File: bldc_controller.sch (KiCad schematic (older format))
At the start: 147 parts, among them J1 Conn_01x06_Male, J2 Banana_Jack, Q1 FDN340P, Q10 IRLB8721PBF, Q11 IRLB8721PBF, Q2 DMN65D8L-7, Q3 DMN65D8L-7, Q4 2N3904, Q5 IRF4905, Q6 IRLB8721PBF, Q7 IRLB8721PBF, Q8 IRLB8721PBF, Q9 IRLB8721PBF, SW1 1301.9314, SW2 D6C40 F1 LFS, SW3 D6C40 F1 LFS, U1 ATmega328P-PU, U10 IRS2004, U2 74LVC2G08, U3 uA7810, U4 LM7805_TO220, U5 CD4044BE, U6 LM339, U7 MCP601-xP, U8 IRS2004, U9 IRS2004, Y1 9B-16.000MBBK-B

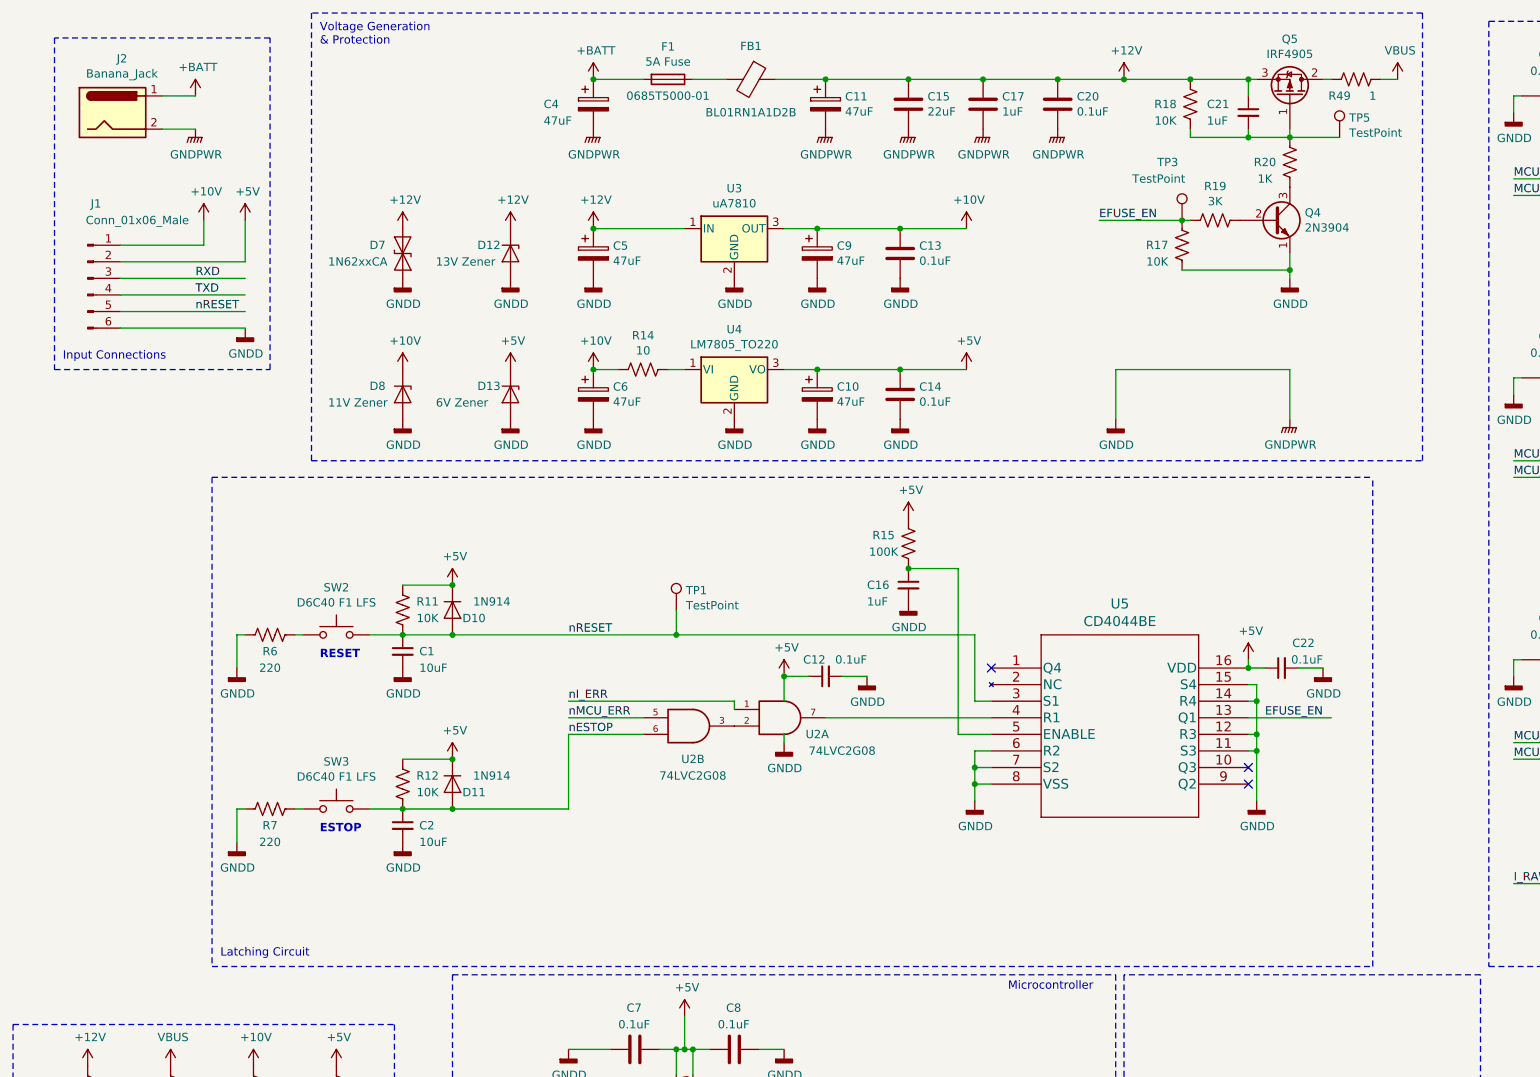
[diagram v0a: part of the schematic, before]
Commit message: Ready for Layout
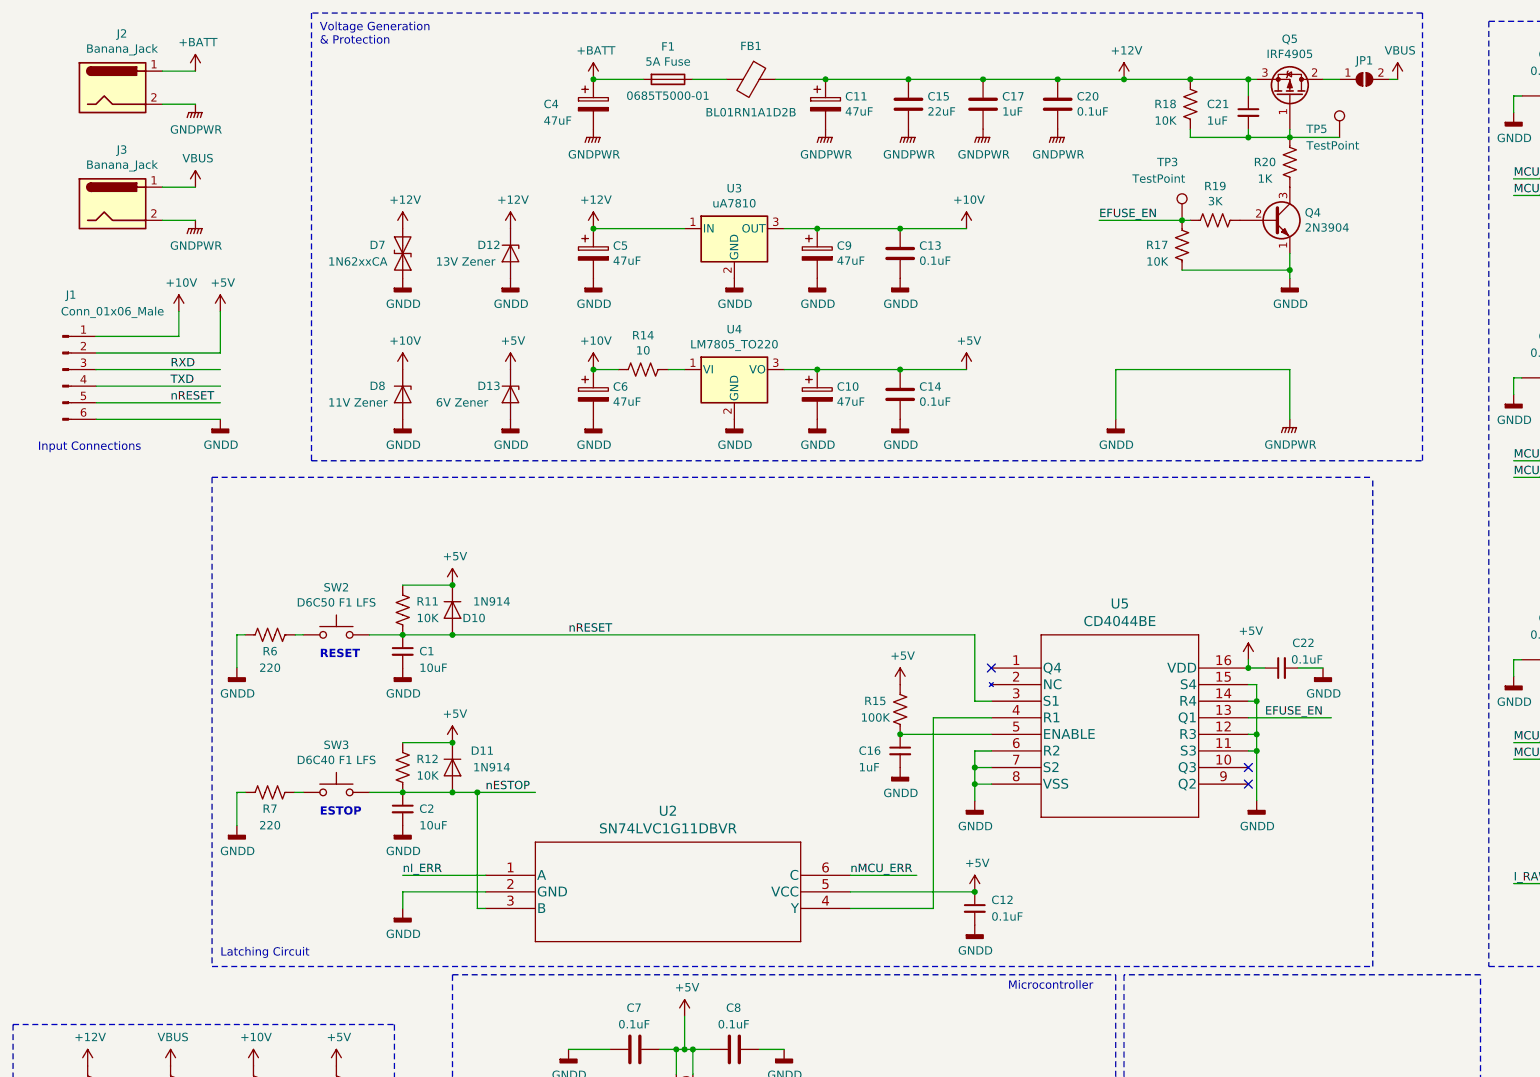
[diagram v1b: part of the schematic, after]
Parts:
- removed R49: 1, symbol Device:R_US
- removed TP1: TestPoint, symbol Connector:TestPoint
- removed U2: 74LVC2G08, symbol 74xGxx:74LVC2G08
- added J3: Banana_Jack, TestPoint:TestPoint_THTPad_D4.0mm_Drill2.0mm, symbol Connector:Barrel_Jack
- added JP1: SolderJumper_2_Open, Jumper:Solder_Jumper_2_Pin_5A, symbol Jumper:SolderJumper_2_Open
- added U2: SN74LVC1G11DBVR, Package_TO_SOT_SMD:SOT-23-6_Handsoldering, symbol SN74LVC1G11DBVR:SN74LVC1G11DBVR
- C1, C12, C13, C14, C15, C16, C17, C18, C19, C2, C20, C21, C22, C23, C24, C25, C26, C27, C28, C29, C3, C30, C31, C32, C33, C7, C8: footprint (none) -> Capacitor_SMD:C_0805_2012Metric_Pad1.15x1.40mm_HandSolder
- C10, C11, C4, C5, C6, C9: footprint (none) -> Capacitor_THT:CP_Radial_D10.0mm_P5.00mm
- D1, D2, D3, D4, D5, D6, D9: footprint (none) -> LED_SMD:LED_0805_2012Metric_Pad1.15x1.40mm_HandSolder
- D12, D13, D8: footprint (none) -> Diode_THT:D_DO-35_SOD27_P7.62mm_Horizontal
- F1: footprint (none) -> Fuse:Fuse_1206_3216Metric_Pad1.42x1.75mm_HandSolder
- FB1: footprint (none) -> Ferrite_THT:Ferrite_Bead_TH
- J1: footprint (none) -> Connector_PinHeader_2.54mm:PinHeader_1x06_P2.54mm_Vertical
- J2: footprint (none) -> TestPoint:TestPoint_THTPad_D4.0mm_Drill2.0mm
- Q1, Q2, Q3: footprint (none) -> Package_TO_SOT_SMD:SOT-23
- R1, R10, R11, R12, R13, R14, R15, R16, R17, R18, R19, R2, R20, R22, R23, R26, R27, R28, R3, R31, R32, R33, R34, R35, R36, R37, R38, R39, R4, R40, R41, R42, R43, R44, R45, R46, R47, R48, R5, R6, R7, R8, R9, RV1: footprint (none) -> Resistor_SMD:R_0805_2012Metric_Pad1.15x1.40mm_HandSolder
- R21, R24, R25, R29, R30: footprint (none) -> Resistor_THT:Power_Resistor_TH
- SW1: footprint (none) -> Button_Switch_SMD:Tactile_Switch_SM
- SW2: value D6C40 F1 LFS -> D6C50 F1 LFS; footprint (none) -> Button_Switch_THT:Pushbutton_Switch_TH
- SW3: footprint (none) -> Button_Switch_THT:Pushbutton_Switch_TH
- TP10, TP11, TP12, TP13, TP14, TP15, TP16, TP17, TP18, TP19, TP2, TP3, TP4, TP5, TP6, TP7, TP8, TP9: footprint (none) -> TestPoint:TestPoint_THTPad_1.0x1.0mm_Drill0.5mm
- U10, U8, U9: footprint (none) -> Package_DIP:DIP-8-16_W7.62mm
- U3: footprint (none) -> Package_TO_SOT_THT:TO-220-3_Vertical
- U5: footprint N16 -> Package_DIP:DIP-16_W7.62mm
- U6: footprint (none) -> Package_DIP:DIP-14_W7.62mm
- Y1: footprint (none) -> Crystal:Crystal_16MHz_TH
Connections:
- wire segments 292 -> 291
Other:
- moved on the sheet: C12, C16, C2, D11, J1, J2, R12, R15, R7, SW3

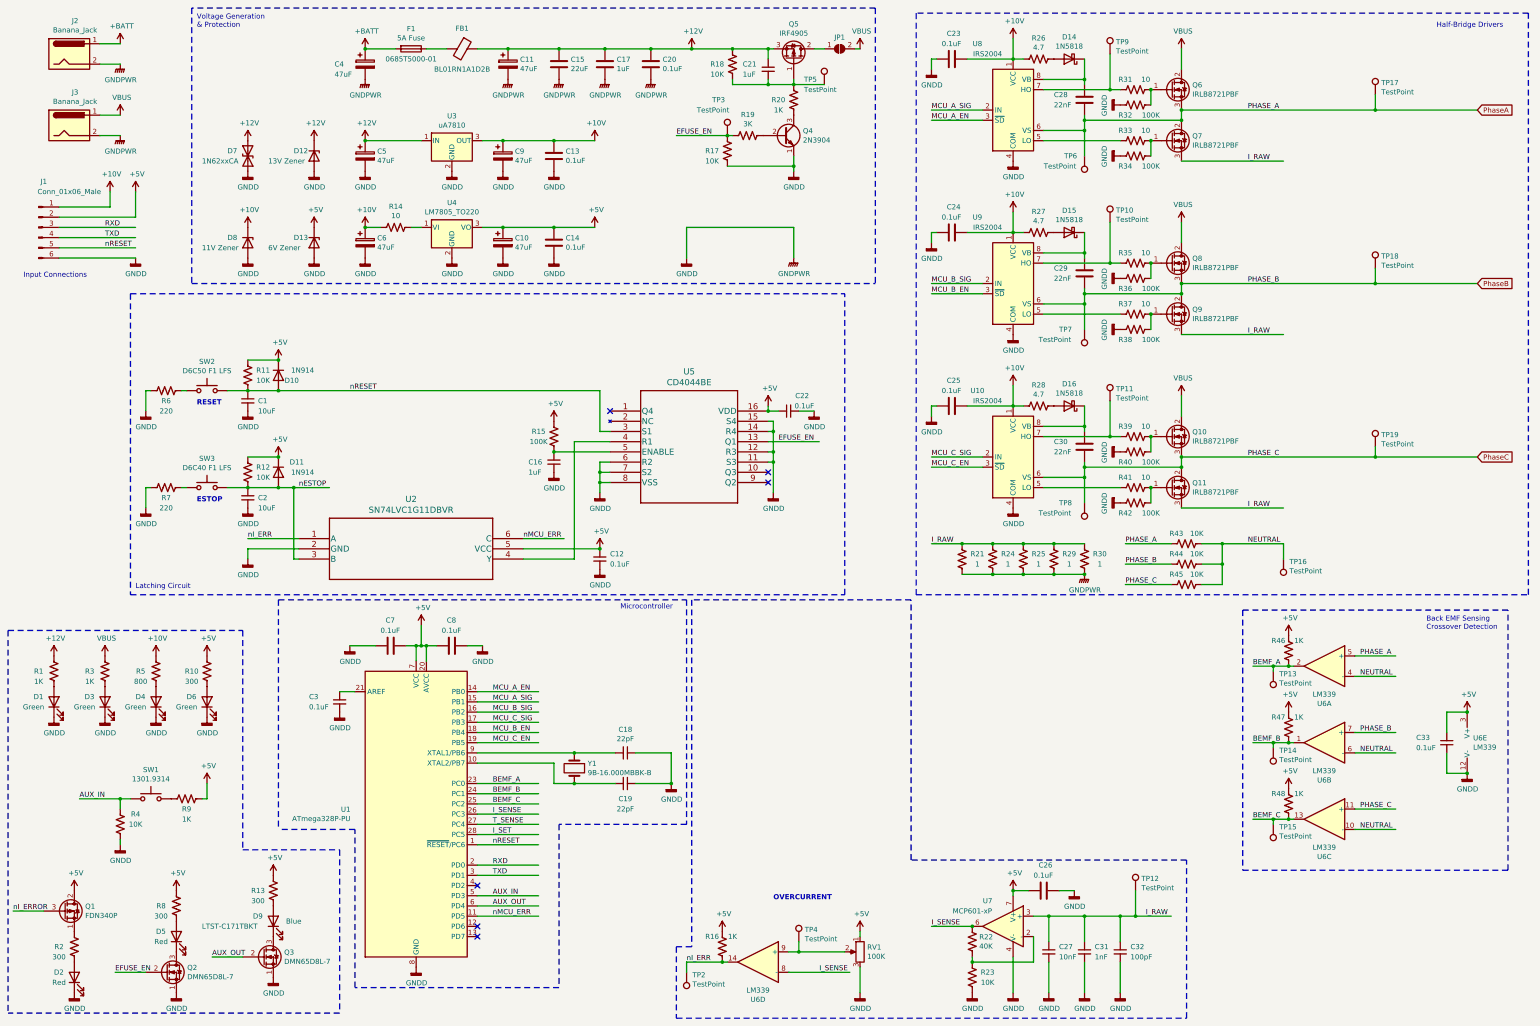
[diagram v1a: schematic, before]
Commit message: Ready to Route
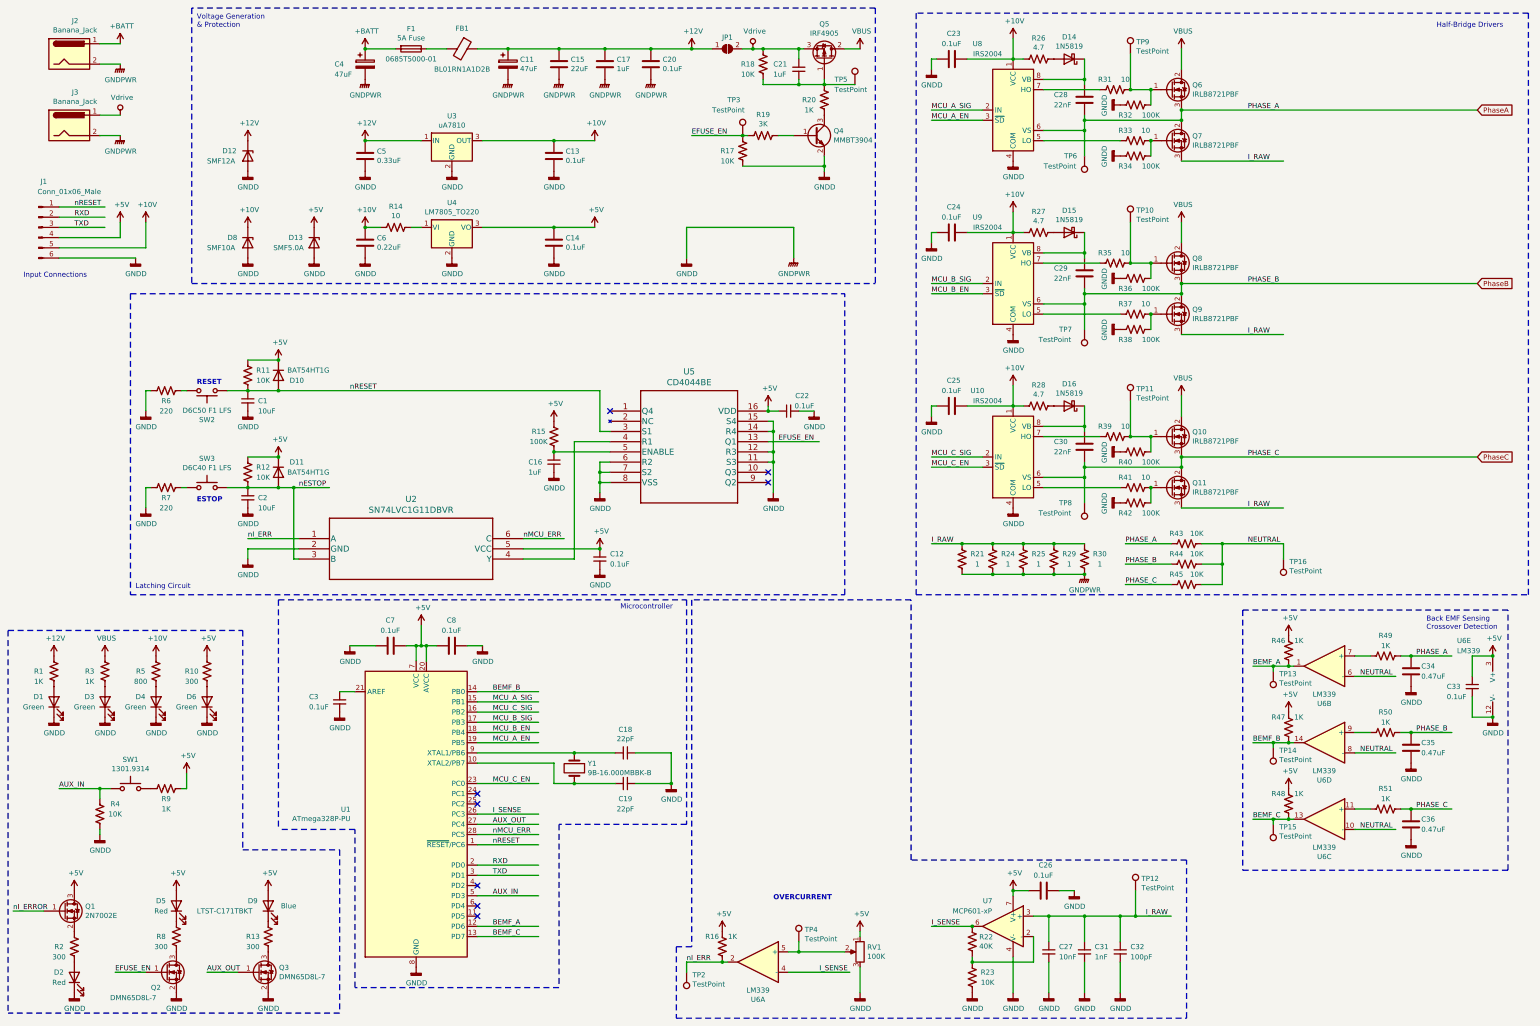
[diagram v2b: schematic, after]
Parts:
- removed C10, C5, C6, C9: 47uF, Capacitor_THT:CP_Radial_D10.0mm_P5.00mm, symbol Device:CP
- removed D7: 1N62xxCA, Diode_THT:D_DO-201AE_P15.24mm_Horizontal, symbol Diode:1N62xxCA
- removed Q1: FDN340P, Package_TO_SOT_SMD:SOT-23, symbol Device:Q_PMOS_SDG
- removed Q2, Q3: DMN65D8L-7, Package_TO_SOT_SMD:SOT-23, symbol Device:Q_NMOS_SGD
- removed Q4: 2N3904, Package_TO_SOT_THT:TO-92_Inline, symbol Transistor_BJT:2N3904
- removed TP17, TP18, TP19: TestPoint, TestPoint:TestPoint_THTPad_1.0x1.0mm_Drill0.5mm, symbol Connector:TestPoint
- added C34, C35, C36: 0.47uF, Capacitor_SMD:C_0805_2012Metric_Pad1.15x1.40mm_HandSolder, symbol Device:C
- added C5: 0.33uF, Capacitor_SMD:C_0805_2012Metric_Pad1.15x1.40mm_HandSolder, symbol Device:C
- added C6: 0.22uF, Capacitor_SMD:C_0805_2012Metric_Pad1.15x1.40mm_HandSolder, symbol Device:C
- added Q1: 2N7002E, Package_TO_SOT_SMD:SOT-23, symbol Transistor_FET:2N7002E
- added Q2, Q3: DMN65D8L-7, Package_TO_SOT_SMD:SOT-23, symbol Transistor_FET:DMN67D7L
- added Q4: MMBT3904, Package_TO_SOT_SMD:SOT-23, symbol Transistor_BJT:MMBT3904
- added R49, R50, R51: 1K, Resistor_SMD:R_0805_2012Metric_Pad1.15x1.40mm_HandSolder, symbol Device:R_US
- D10, D11: value 1N914 -> BAT54HT1G; footprint Diode_THT:D_DO-35_SOD27_P7.62mm_Horizontal -> Diode_SMD:D_SOD-323_HandSoldering
- D12: value 13V Zener -> SMF12A; footprint Diode_THT:D_DO-35_SOD27_P7.62mm_Horizontal -> Diode_SMD:D_SOD-123F
- D13: value 6V Zener -> SMF5.0A; footprint Diode_THT:D_DO-35_SOD27_P7.62mm_Horizontal -> Diode_SMD:D_SOD-123F
- D14, D15, D16: value 1N5818 -> 1N5819; footprint Diode_THT:D_DO-41_SOD81_P10.16mm_Horizontal -> Diode_SMD:D_SOD-123
- D8: value 11V Zener -> SMF10A; footprint Diode_THT:D_DO-35_SOD27_P7.62mm_Horizontal -> Diode_SMD:D_SOD-123F
- J2, J3: footprint TestPoint:TestPoint_THTPad_D4.0mm_Drill2.0mm -> Connector_BarrelJack:BarrelJack_CUI_PJ-063AH_Horizontal
- RV1: footprint Resistor_SMD:R_0805_2012Metric_Pad1.15x1.40mm_HandSolder -> Potentiometer_THT:Potentiometer_Bourns_3339P_Vertical_HandSoldering
- U10, U8, U9: footprint Package_DIP:DIP-8-16_W7.62mm -> Package_DIP:DIP-8_W7.62mm
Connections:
- net labels added: Vdrive
- net labels removed: I_SET, T_SENSE
- wire segments 291 -> 289
- no-connect marks 6 -> 8
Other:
- moved on the sheet: C21, C33, D12, D5, D9, JP1, Q5, R13, R17, R18, R19, R20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
